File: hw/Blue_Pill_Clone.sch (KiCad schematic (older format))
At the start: 31 parts, among them J5 USB_B_Micro, J6 Conn_01x04_Male, J7 Conn_02x03_Odd_Even, SW1 SW_Push, U2 MIC5504-3.3YM5, U3 STM32F103C8Tx, Y1 32.768k, Y2 8MHz

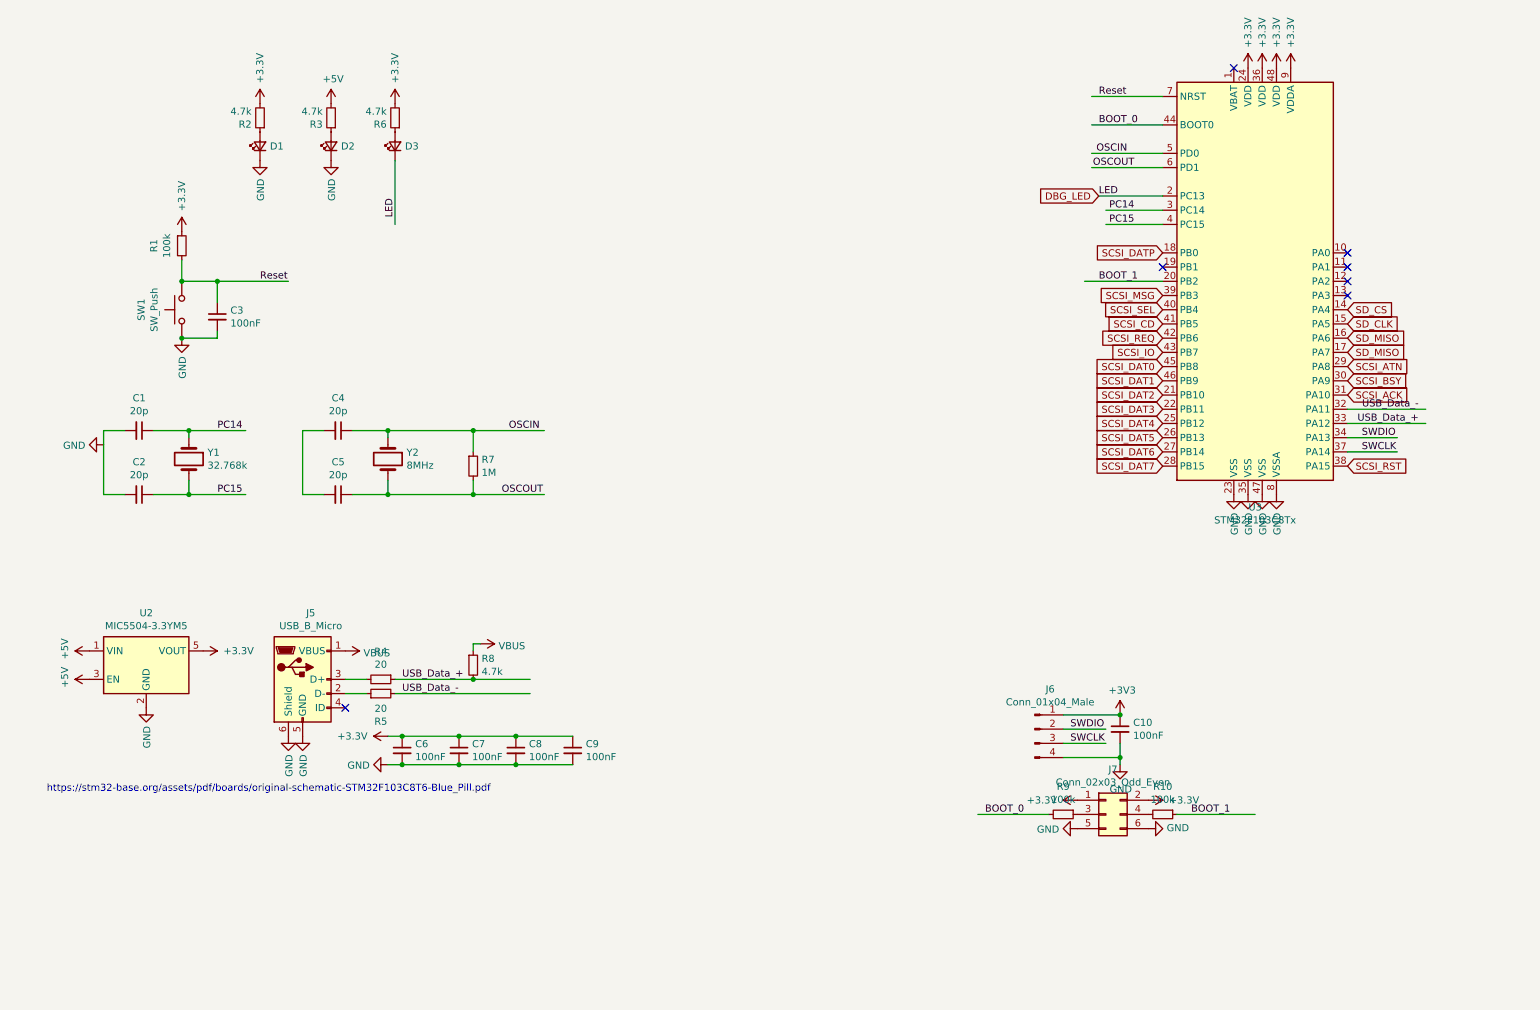
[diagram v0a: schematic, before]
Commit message: Updated bluepill all-in-one
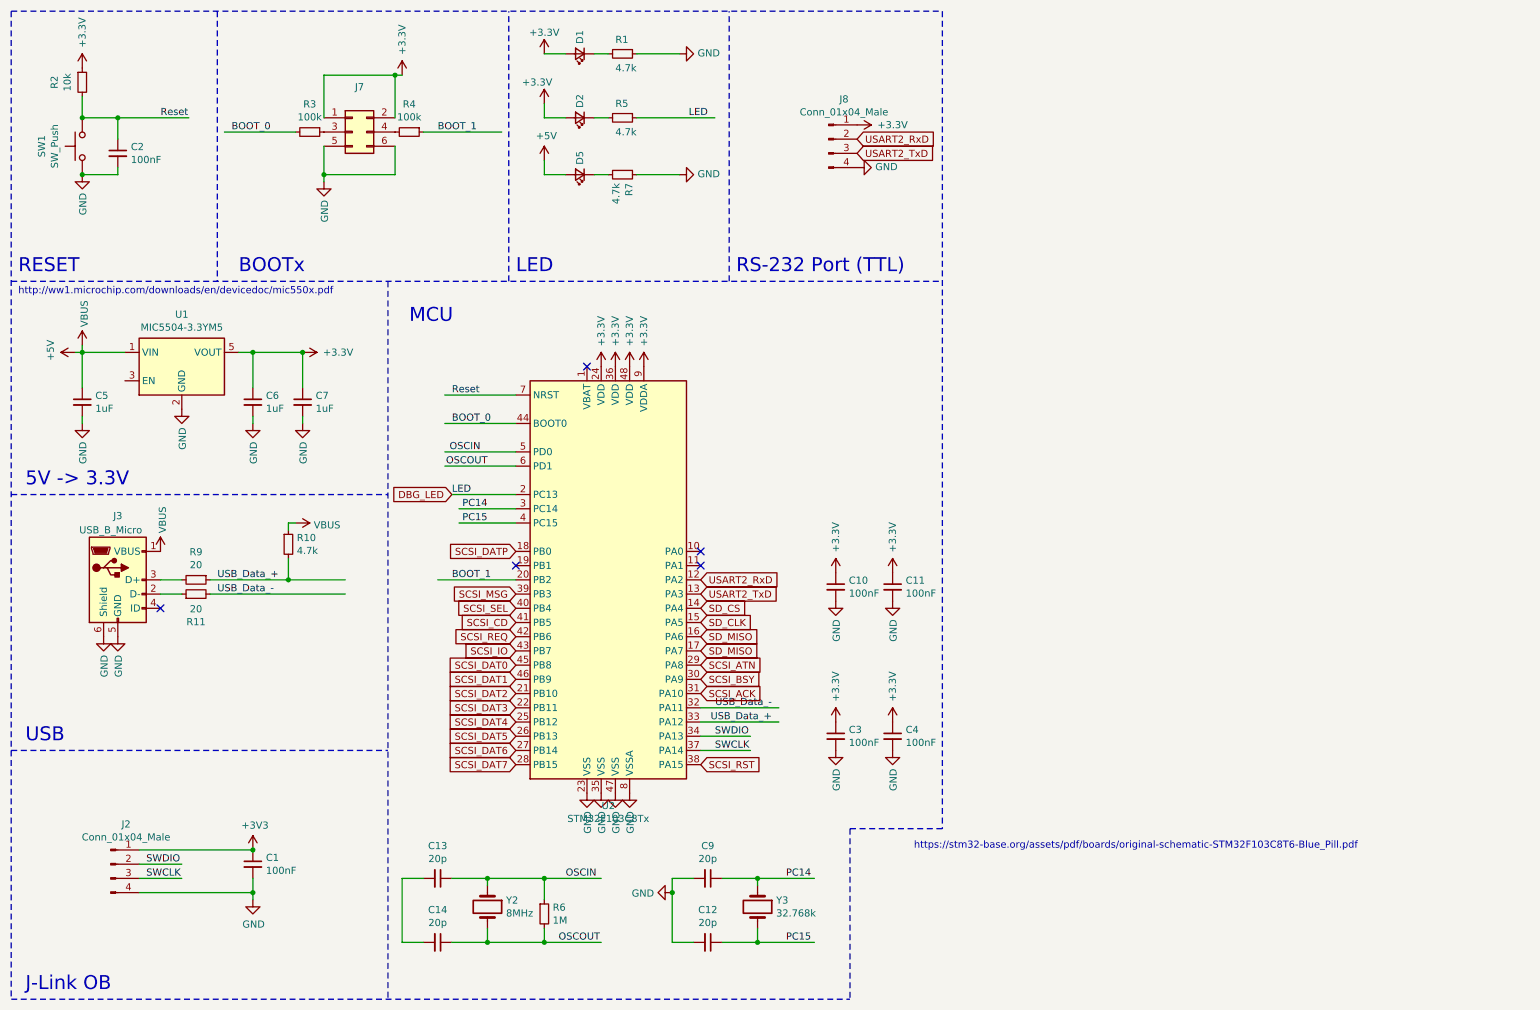
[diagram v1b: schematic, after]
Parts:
- added C5, C6, C7: 1uF, Capacitor_SMD:C_0603_1608Metric, symbol Device:C_Small
- added J8: Conn_01x04_Male, Connector_PinHeader_2.54mm:PinHeader_1x04_P2.54mm_Vertical, symbol Connector:Conn_01x04_Male
- R2: renamed from R1; value 100k -> 10k; LCSC C25803 -> C25804
- SW1: footprint Button_Switch_SMD:SW_SPST_B3S-1000 -> Button_Switch_SMD:SW_SPST_B3U-1000P; LCSC C412369????? -> C231329
- renumbered C10 to C1, C6 to C10, C7 to C11, C2 to C12, C4 to C13, C5 to C14, C3 to C2, C8 to C3, C9 to C4, C1 to C9, D3 to D2, D2 to D5, J6 to J2, J5 to J3, R2 to R1, R8 to R10, R5 to R11, R9 to R3, R10 to R4, R6 to R5, R7 to R6, R3 to R7, R4 to R9, U2 to U1, U3 to U2, Y1 to Y3
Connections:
- net labels added: USART2_RxD, USART2_TxD
- wire segments 64 -> 87
- no-connect marks 7 -> 5
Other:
- note added: "5V -> 3.3V"
- note added: "BOOTx"
- note added: "J-Link OB"
- note added: "LED"
- note added: "MCU"
- note added: "RESET"
- note added: "RS-232 Port (TTL)"
- note added: "USB"
- note added: "http://ww1.microchip.com/downloads/en/devicedoc/mic550x.pdf"
- moved on the sheet: C1, C10, C11, C12, C13, C14, C2, C3, C4, C9, D1, D2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
